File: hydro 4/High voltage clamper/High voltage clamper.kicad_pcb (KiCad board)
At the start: 2 copper layers, 66.9 x 55 mm, 6 parts, among them Q1 IRF740

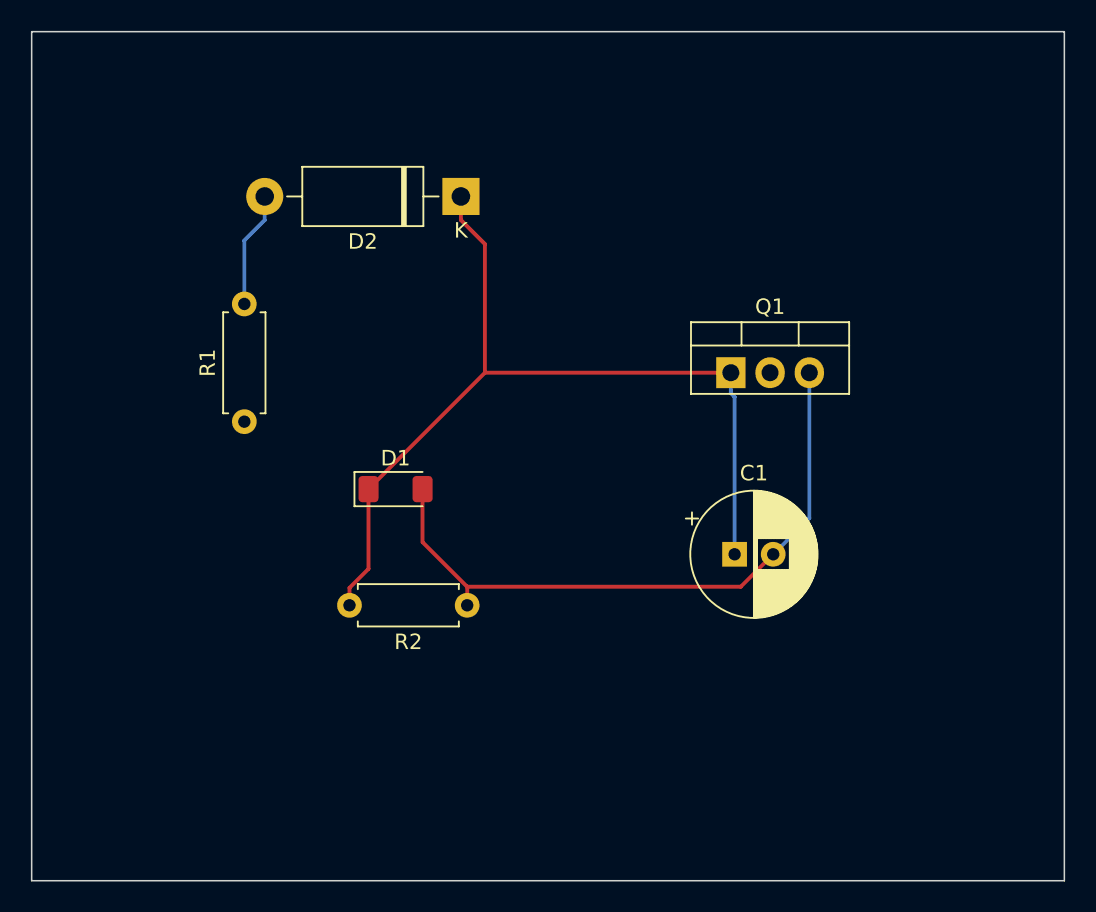
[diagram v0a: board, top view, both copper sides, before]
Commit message: Updated schematic
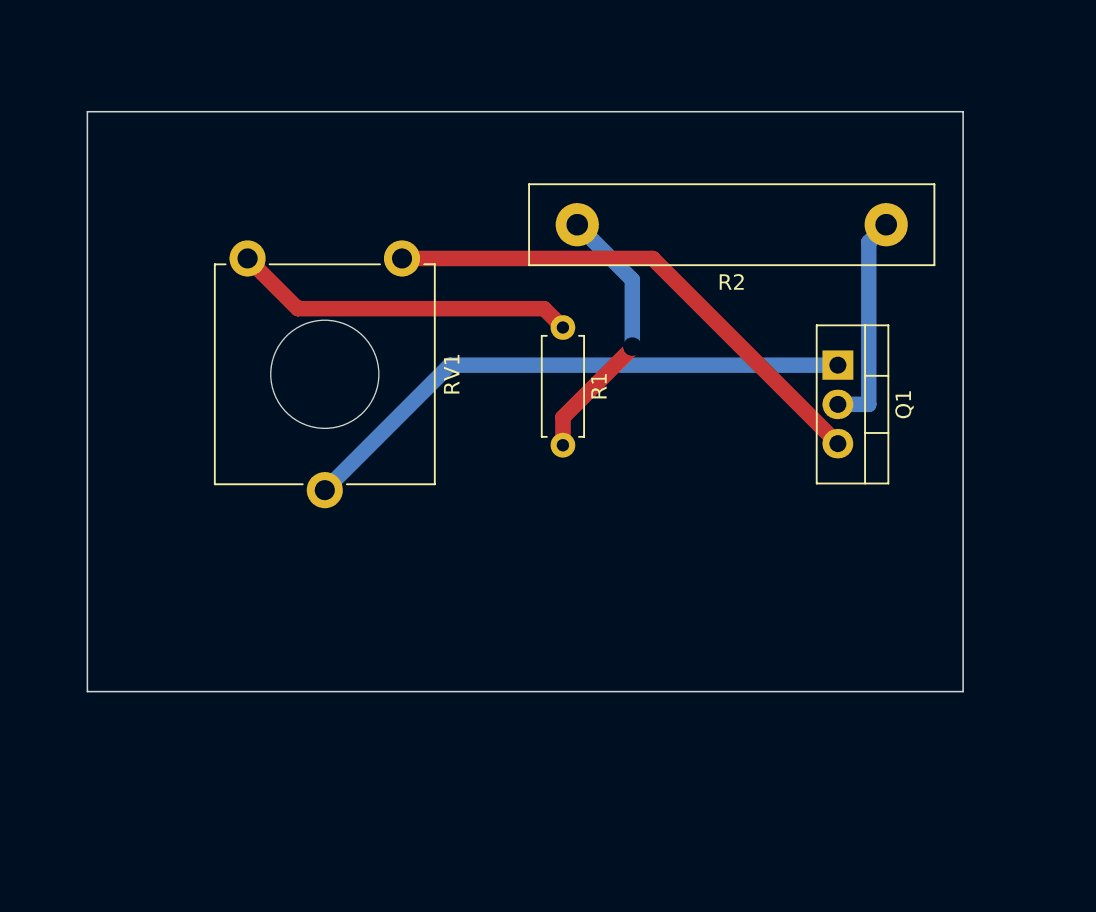
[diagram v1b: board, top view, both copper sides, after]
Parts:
- removed C1: 47uF, Capacitor_THT:CP_Radial_D8.0mm_P2.50mm
- removed D1: ZMDxx, Diode_SMD:D_MiniMELF
- removed D2: D, Diode_THT:D_DO-15_P12.70mm_Horizontal
- added RV1: 1M, Potentiometer_THT:Potentiometer_ACP_CA14V-15_Vertical_Hole, F.Cu at (114.8, 81.1)
- R1: value 10k -> 4.7M
- R2: value 100k -> 50 200watt; footprint Resistor_THT:R_Axial_DIN0207_L6.3mm_D2.5mm_P7.62mm_Horizontal -> Resistor_THT:R_Box_L26.0mm_W5.0mm_P20.00mm
- moved R2 36.6 mm to (156.1, 78.9)
- moved R1 21.5 mm to (135.2, 85.6), turned to -90 degrees
- moved Q1 6.95 mm to (153.0, 88.0), turned to -90 degrees
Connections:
- Q1 pad 1: Net-(D1-K) -> Net-(Q1-G)
- Q1 pad 2: Net-(LA1--) -> Net-(Q1-D)
- R1 pad 1: +VDC -> Net-(R1-Pad1)
- R1 pad 2: Net-(D2-A) -> +VDC
- R2 pad 1: -VDC -> Net-(Q1-D)
- R2 pad 2: Net-(D1-K) -> +VDC
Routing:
- net Net-(D1-K): track 58.5 -> 0.00 mm
- net Net-(Q1-G): track 0.00 -> 36.6 mm
- net Net-(R1-Pad1): track 0.00 -> 22.3 mm
- net +VDC: track 0.00 -> 17.6 mm, vias 0 -> 1
- net Net-(Q1-D): track 0.00 -> 14.1 mm
- net -VDC: track 42.1 -> 33.2 mm
- net Net-(D2-A): track 7.51 -> 0.00 mm
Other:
- board size 66.9 x 55 mm -> 56.7 x 37.5 mm
